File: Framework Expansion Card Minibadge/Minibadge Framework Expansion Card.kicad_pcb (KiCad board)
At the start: 2 copper layers, 26 x 54.5 mm, 14 parts, among them P1 Connector_USB_C_Plug_USB2.0, U1 AP2112K-3.3

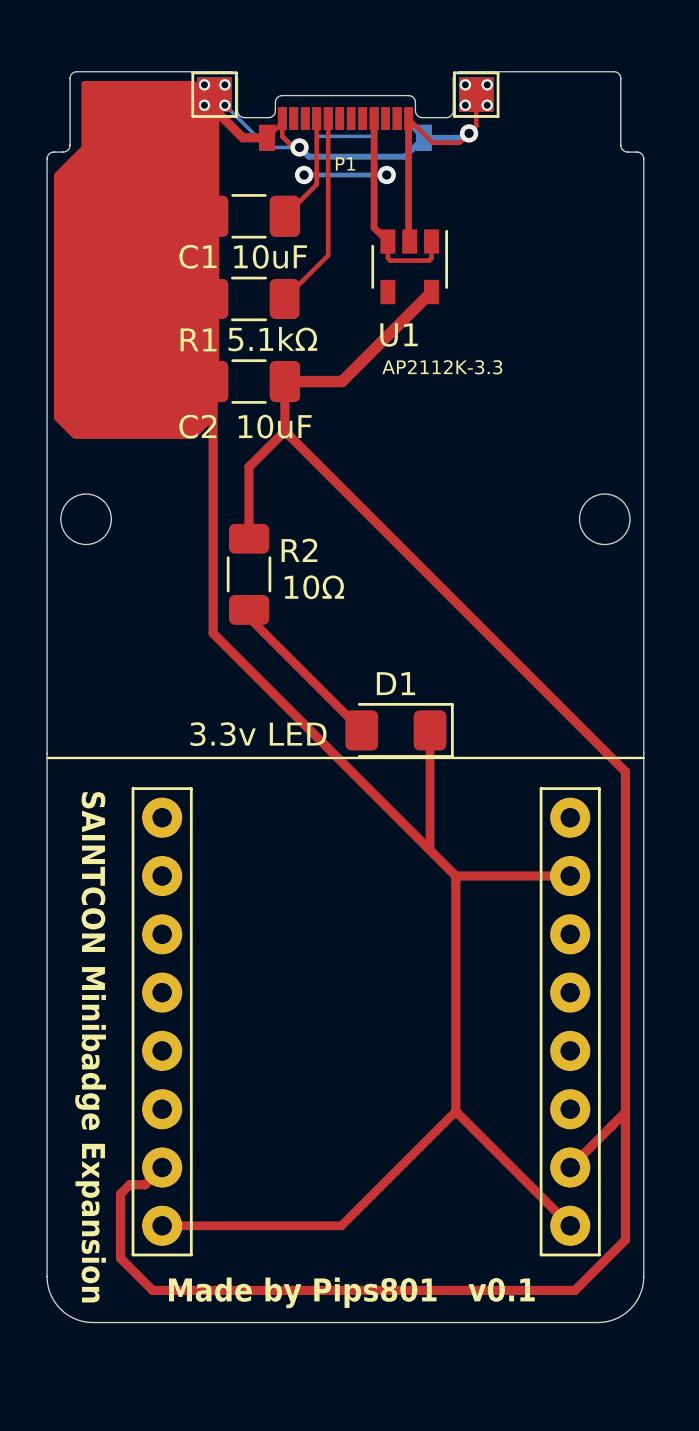
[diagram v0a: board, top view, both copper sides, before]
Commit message: Add files via upload
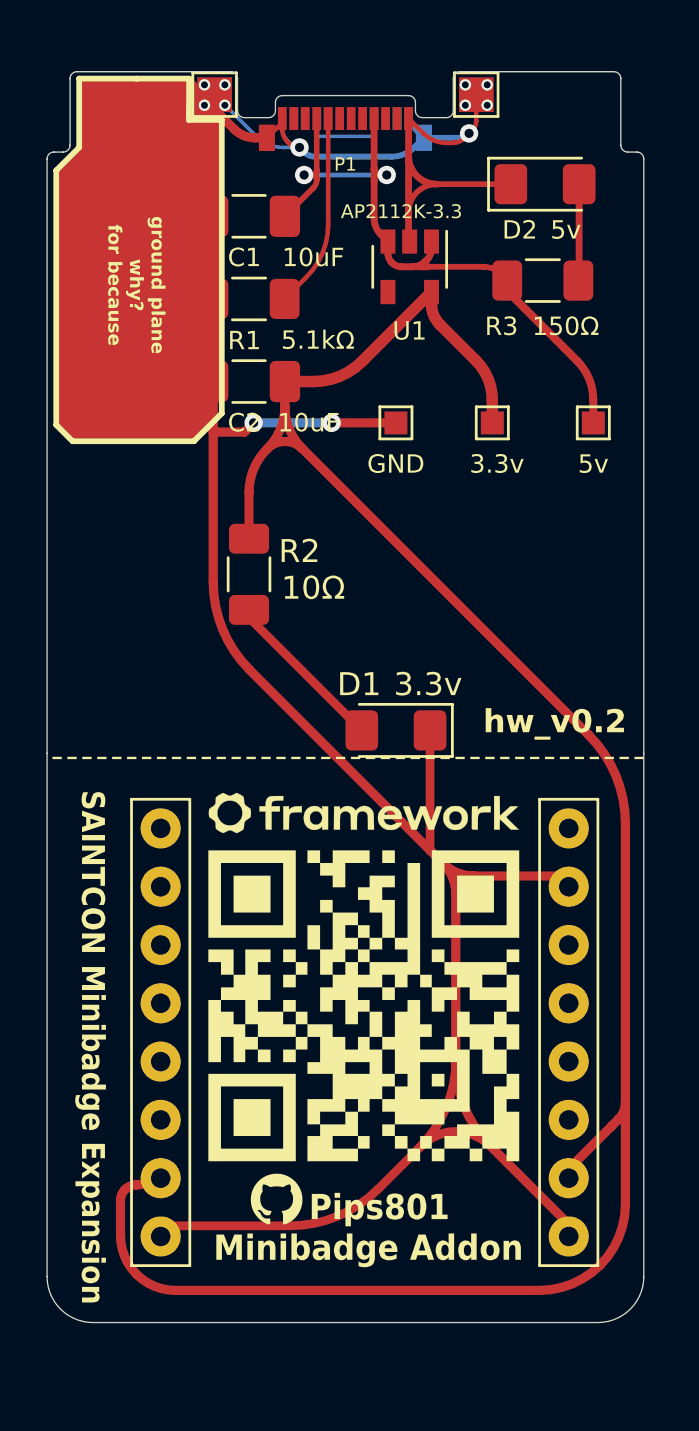
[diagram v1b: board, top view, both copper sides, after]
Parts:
- removed H1, H2: MountingHole, MountingHole:MountingHole_2.2mm_M2
- added ?: , LOGO, F.Cu at (133.8, 140.4)
- added ?: , Expansion_Card:Framework-Logo_1.5mm_SilkScreen, F.Cu at (133.8, 132.0)
- added ?: , LOGO, F.Cu at (130.0, 148.8)
- added D2: LED_Red, LED_SMD:LED_1206_3216Metric_Pad1.42x1.75mm_HandSolder, F.Cu at (141.7, 104.6)
- added R3: 150Ω, Resistor_SMD:R_1206_3216Metric_Pad1.30x1.75mm_HandSolder, F.Cu at (141.6, 108.8)
- added TP5: Connector_TestPoint_VBUS+, TestPoint:TestPoint_Pad_1.0x1.0mm, F.Cu at (143.8, 115.0)
- added TP6: Connector_TestPoint_3.3v, TestPoint:TestPoint_Pad_1.0x1.0mm, F.Cu at (139.4, 115.0)
- added TP7: Connector_TestPoint_GND, TestPoint:TestPoint_Pad_1.0x1.0mm, F.Cu at (135.2, 115.0)
- D1: value LED_R -> LED_Red
- TP1, TP2, TP3, TP4: value Connector_TestPoint -> Connector_TestPoint_GND
- moved MB1 0.47 mm to (144.0, 131.4)
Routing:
- net /GND: track 114.8 -> 136.0 mm, vias 10 -> 12
- net /VBUS+: track 22.6 -> 36.2 mm
- net /+3V3: track 88.9 -> 97.8 mm
- net Net-(D2-A): track 0.00 -> 4.21 mm
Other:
- board text added: "150Ω"
- board text added: "3.3v"
- board text added: "5v"
- board text added: "GND"
- board text added: "Ground plane for because"
- board text added: "Pips801 Minibadge Addon"
- board text added: "ground plane why? for because"
- board text added: "hw_v0.2"
- board text added: "insert graphic here"
- board text removed: "3.3v LED"
- board text removed: "Made by Pips801 v0.1"
- board text removed: "insert grapgic here"
